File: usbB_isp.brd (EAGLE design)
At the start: 100 x 80 mm, 12 parts, among them IC1 788TV, IC2 TINY13-20PU, X1 PN61729-S

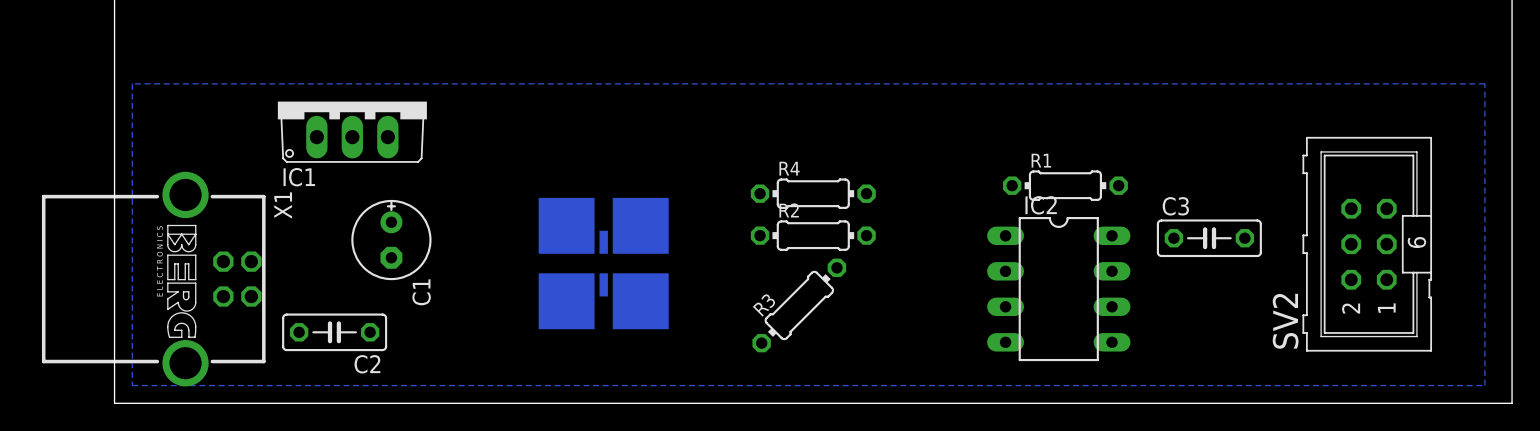
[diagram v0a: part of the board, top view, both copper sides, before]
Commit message: routing
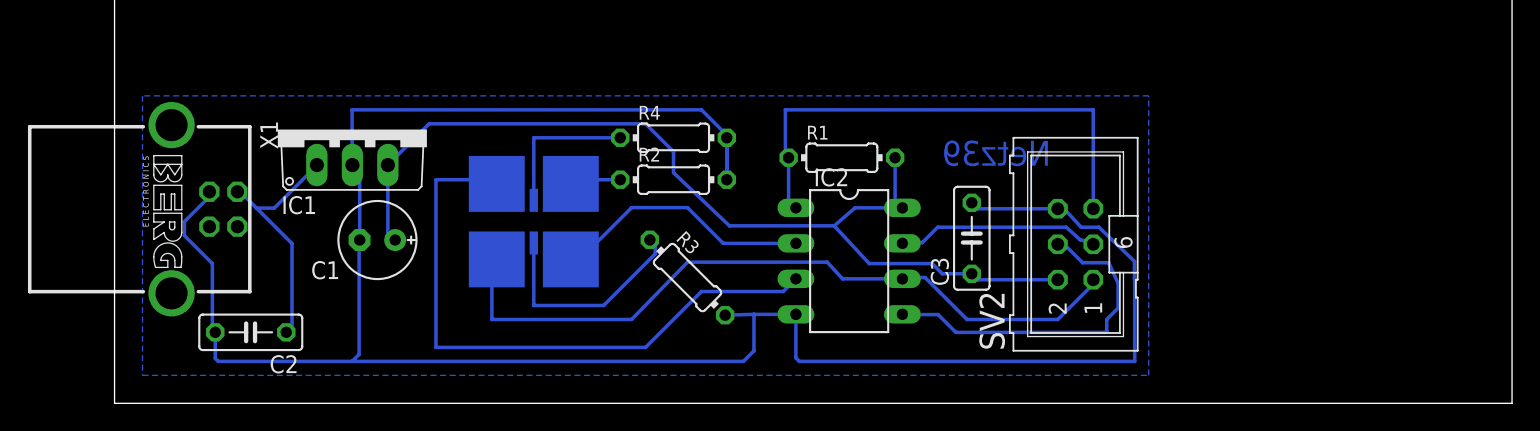
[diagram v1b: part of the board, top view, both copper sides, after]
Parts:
- moved SV2 21.0 mm to (68.8, 11.4)
- moved C3 17.0 mm to (61.3, 11.8), turned to 90 degrees
- moved R1 16.1 mm to (52.0, 17.6)
- moved IC2 15.1 mm to (52.6, 10.2)
- moved R2 10.8 mm to (40.0, 16.0)
- moved R4 10.8 mm to (40.0, 19.0)
- moved R3 8.25 mm to (41.0, 9.00), turned to 315 degrees
- moved C2 6.00 mm to (9.75, 5.08)
- moved LED1 5.83 mm to (30.0, 13.0)
- moved X1 5.10 mm to (4.08, 13.9)
- moved IC1 2.00 mm to (17.0, 19.6)
- moved C1 1.00 mm to (18.8, 11.7), turned to 180 degrees
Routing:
- net GND: track 0.00 -> 160.4 mm
- net VCC: track 0.00 -> 69.4 mm
- net MISO: track 0.00 -> 52.4 mm
- net N$9: track 0.00 -> 46.3 mm
- net _RESET: track 0.00 -> 36.6 mm
- net N$10: track 0.00 -> 24.8 mm
- net N$3: track 0.00 -> 20.2 mm
- net N$1: track 0.00 -> 17.9 mm
- net N$7: track 0.00 -> 16.1 mm
- net SCK: track 0.00 -> 14.6 mm
- net N$6: track 0.00 -> 10.7 mm
- net N$8: track 0.00 -> 6.11 mm
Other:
- board text added: "Netz39"
